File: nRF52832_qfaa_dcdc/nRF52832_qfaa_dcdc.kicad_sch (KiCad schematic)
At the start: 20 parts, among them U1 NRF52832, X1 32MHz, X2 32.768kHz

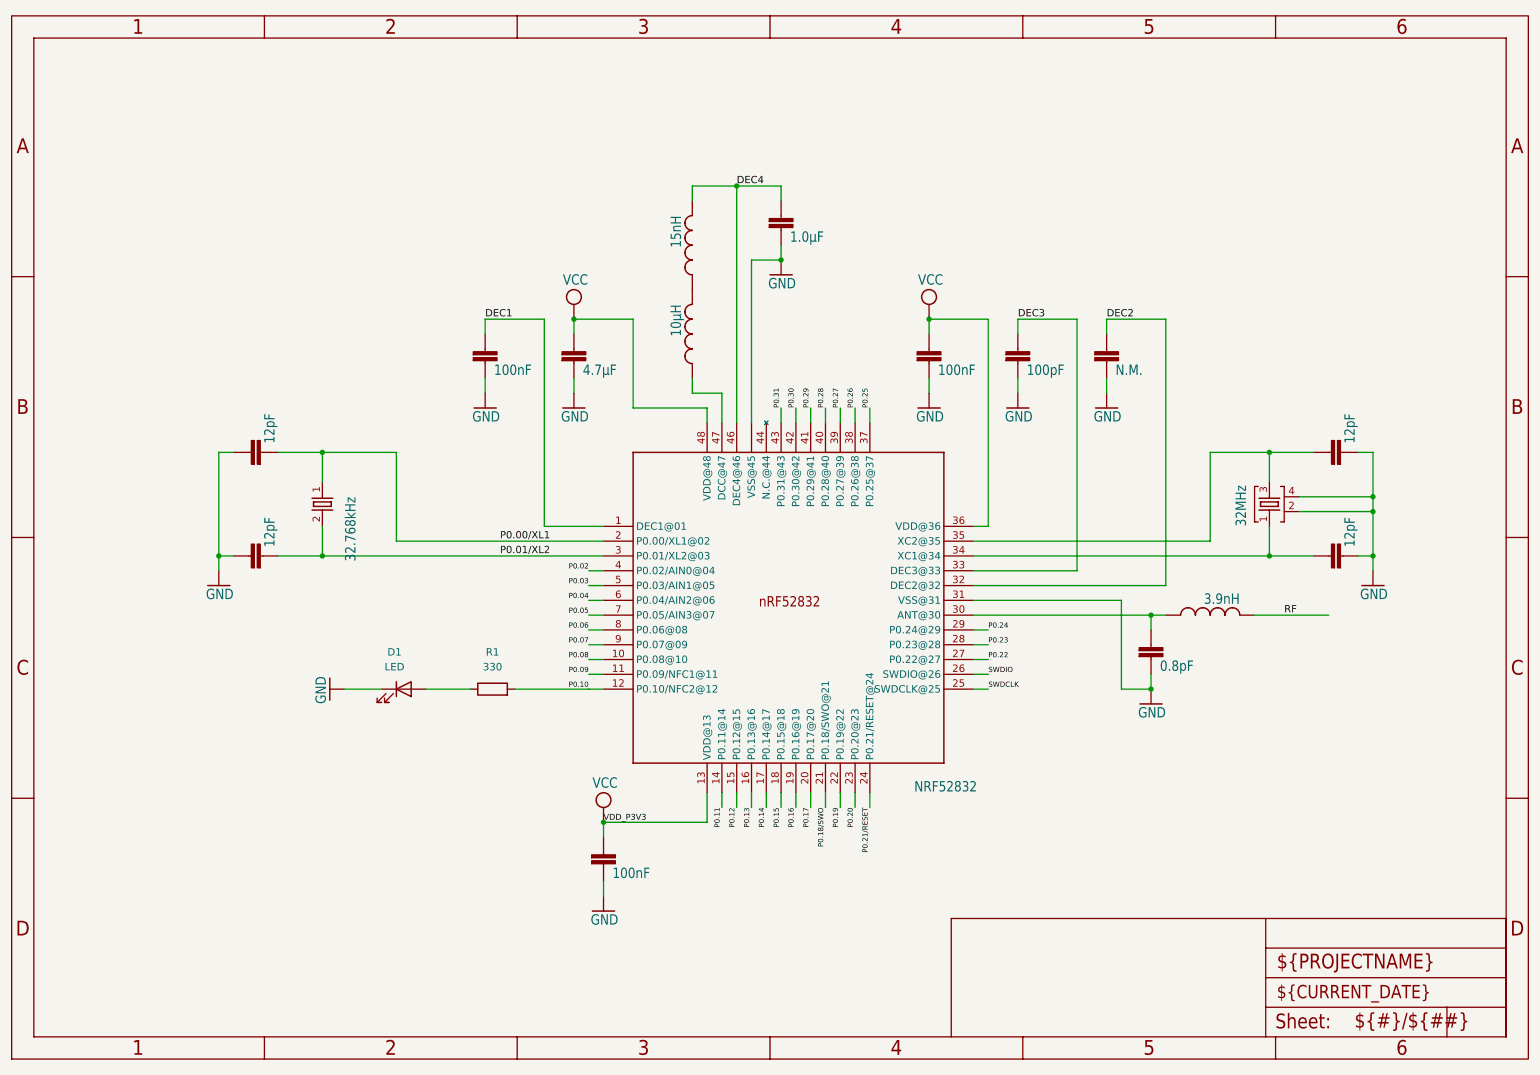
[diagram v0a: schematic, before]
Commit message: commit changement elec
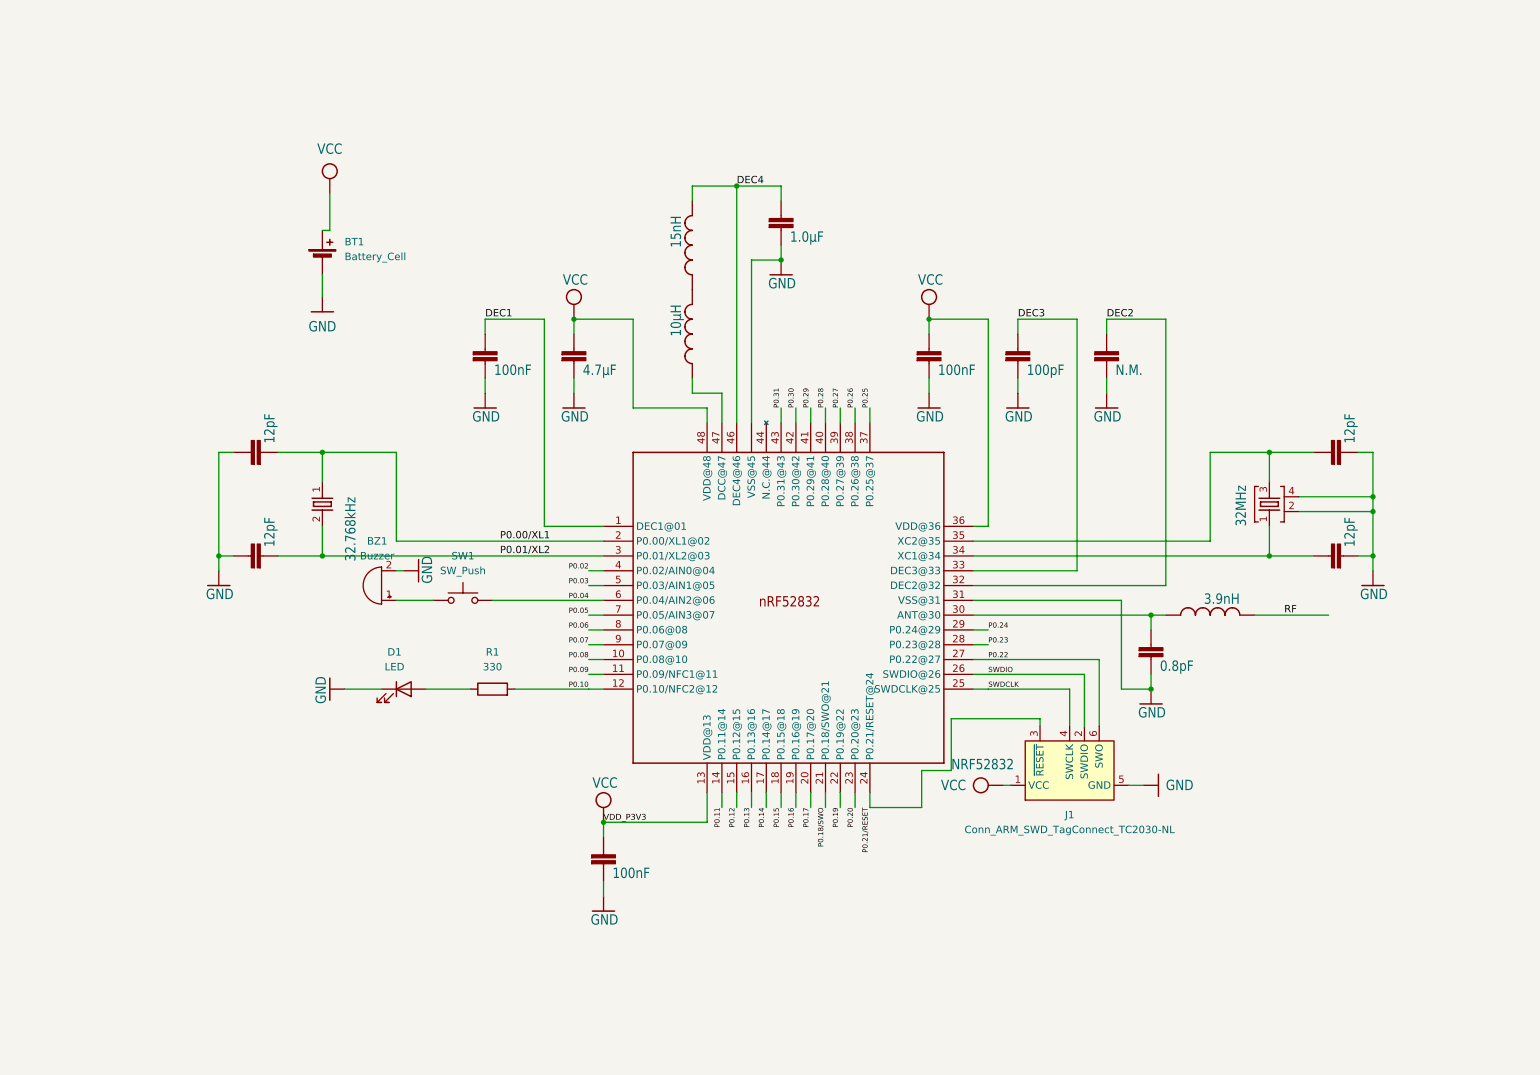
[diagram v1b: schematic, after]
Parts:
- added BT1: Battery_Cell, Buzzer_Beeper:Buzzer_Mallory_AST1240MLQ, symbol Device:Battery_Cell
- added BZ1: Buzzer, Buzzer_Beeper:Buzzer_Mallory_AST1240MLQ, symbol Device:Buzzer
- added J1: Conn_ARM_SWD_TagConnect_TC2030-NL, Connector:Tag-Connect_TC2030-IDC-NL_2x03_P1.27mm_Vertical, symbol Connector:Conn_ARM_SWD_TagConnect_TC2030-NL
- added SW1: SW_Push, Button_Switch_THT:SW_CW_GPTS203211B, symbol Switch:SW_Push
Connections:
- net GND: now also BT1.2 (-), BZ1.2 (+), J1.5 (GND)
- net P0.04: now also SW1.2
- net P0.21/RESET: now also J1.3 (~{RESET})
- net P0.22: now also J1.6 (SWO)
- net SWDCLK: now also J1.4 (SWCLK)
- net SWDIO: now also J1.2 (SWDIO)
- net VCC: now also BT1.1 (+), J1.1 (VCC)
- new net: BZ1.1 (-), SW1.1
